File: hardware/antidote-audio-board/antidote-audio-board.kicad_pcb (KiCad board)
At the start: 4 copper layers, 65 x 30 mm, 60 parts, among them J1 Cubie GPIO, J2 Instrument Out, J3 Phones, J4 Instrument In, J5 LED Header, J6 I2C Header, SW1 Footswitch, SW2 Footswitch, U1 ADS1115IDGS, U2 MCP6002-xSN, U3 TAC5112IRGER, U4 LP5907MFX-3.3

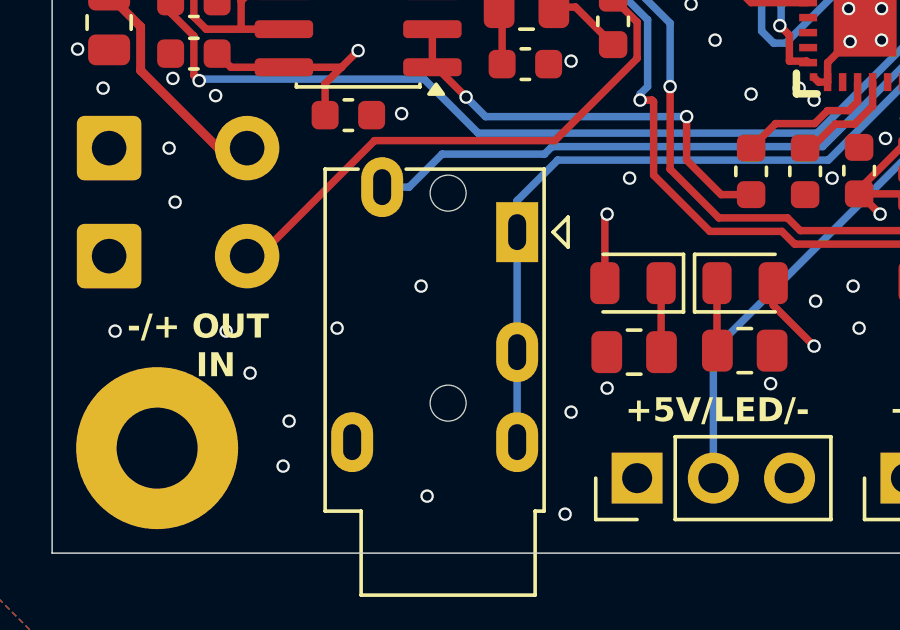
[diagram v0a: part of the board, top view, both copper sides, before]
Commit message: feat: fix schematic issues & document audio bring up
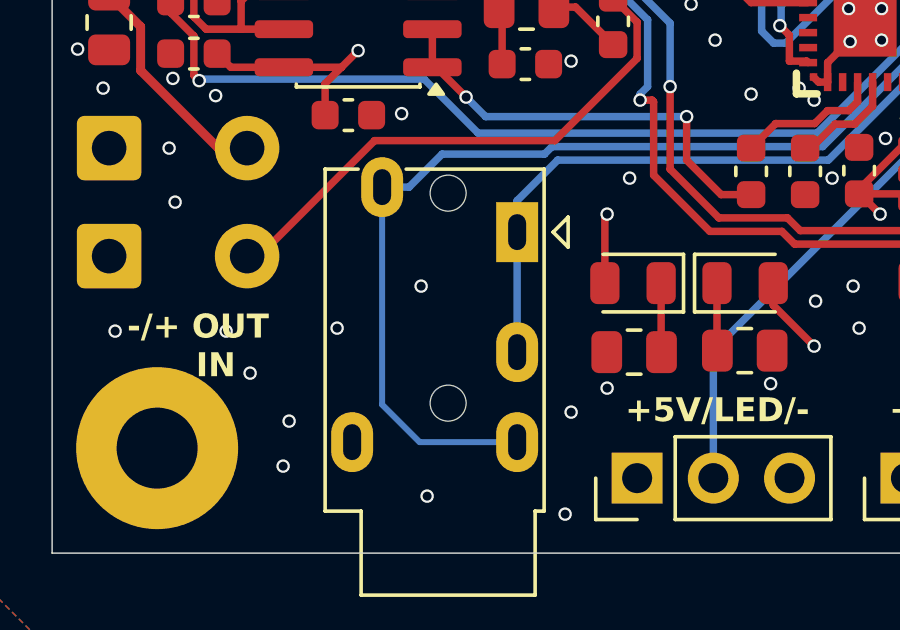
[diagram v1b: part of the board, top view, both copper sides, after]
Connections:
- J3 pad R2: /Phones Mono -> /Phones Sleeve
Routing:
- net /Phones Sleeve: track 25.8 -> 38.1 mm
- net /Phones Mono: track 26.7 -> 23.7 mm
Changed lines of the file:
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@@
 			(layers "*.Cu" "*.Mask")
 			(remove_unused_layers no)
-			(net "/Phones Mono")
+			(net "/Phones Sleeve")
 			(pintype "passive")
 		)
@@
 	)
 	(segment
-		(start 48 58.8)
-		(end 48 55.8)
-		(width 0.25)
-		(layer "B.Cu")
-		(net "/Phones Mono")
-	)
-	(segment
 		(start 58.372792 49.4)
 		(end 49.35 49.4)
@@
 	)
 	(segment
+		(start 44.75 58.8)
+		(end 43.5 57.55)
+		(width 0.2)
+		(layer "B.Cu")
+		(net "/Phones Sleeve")
+	)
+	(segment
 		(start 49.163604 48.95)
 		(end 48.913604 49.2)
@@
 		(layer "B.Cu")
 		(net "/Phones Sleeve")
+	)
+	(segment
+		(start 48 58.8)
+		(end 44.75 58.8)
+		(width 0.2)
+		(layer "B.Cu")
+		(net "/Phones Sleeve")
+	)
+	(segment
+		(start 43.5 57.55)
+		(end 43.5 50.3)
+		(width 0.2)
+		(layer "B.Cu")
+		(net "/Phones Sleeve")
